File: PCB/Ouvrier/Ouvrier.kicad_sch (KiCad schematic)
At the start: 13 parts, among them J1 Batterie, J2 VBAT Xiao, J3 DC 5V input, Q1 2N2222B, U1 XIAO-ESP32-S3-Plus-DIP, U2 BMP581, U3 UWB

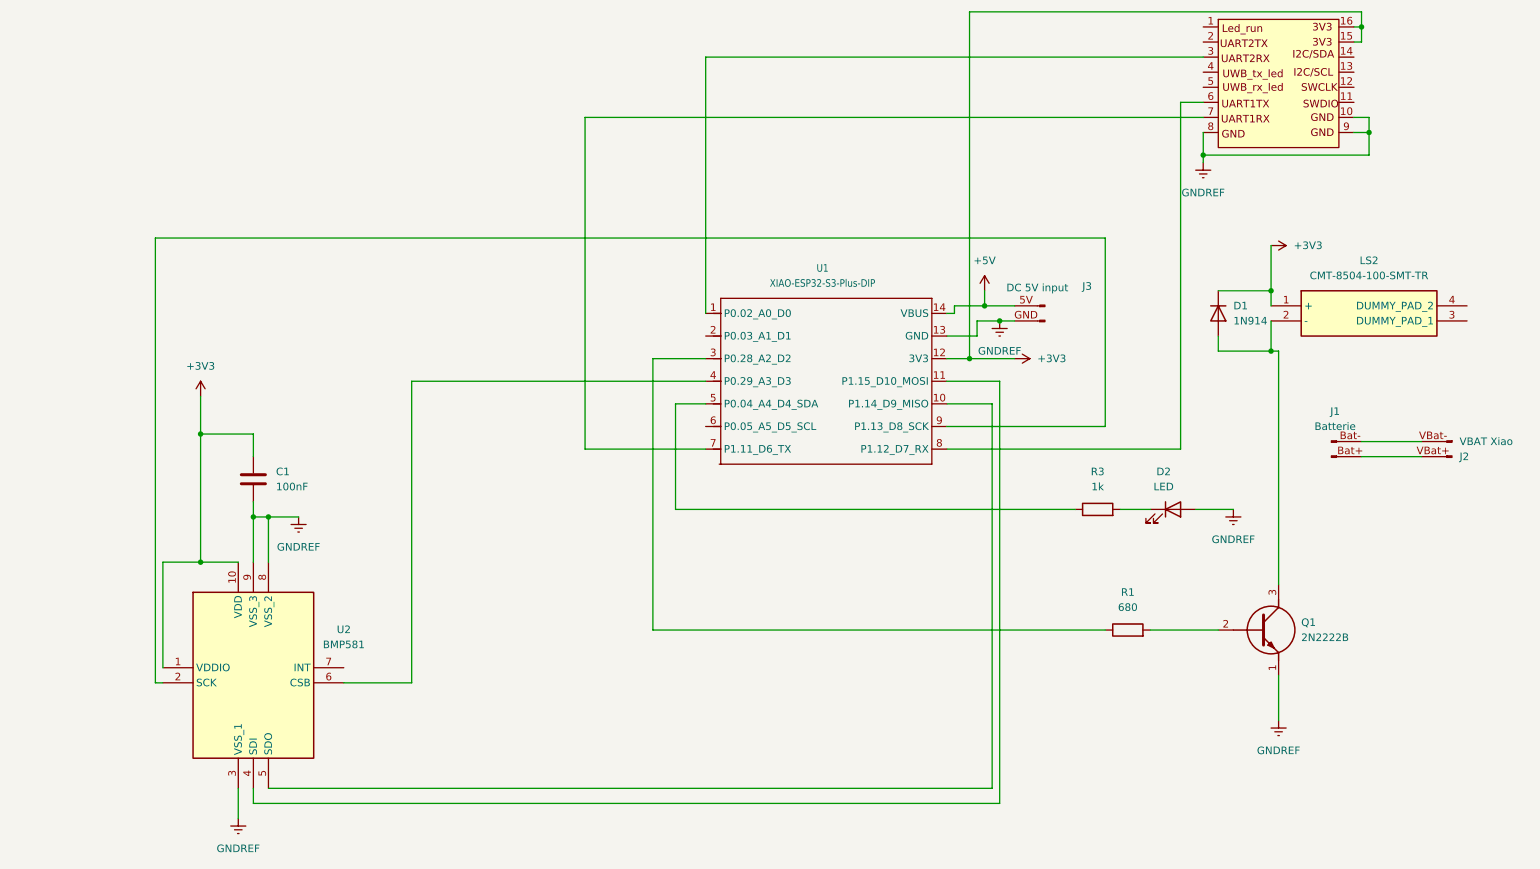
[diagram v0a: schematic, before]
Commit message: Ouvrier_v9_changement_bmp
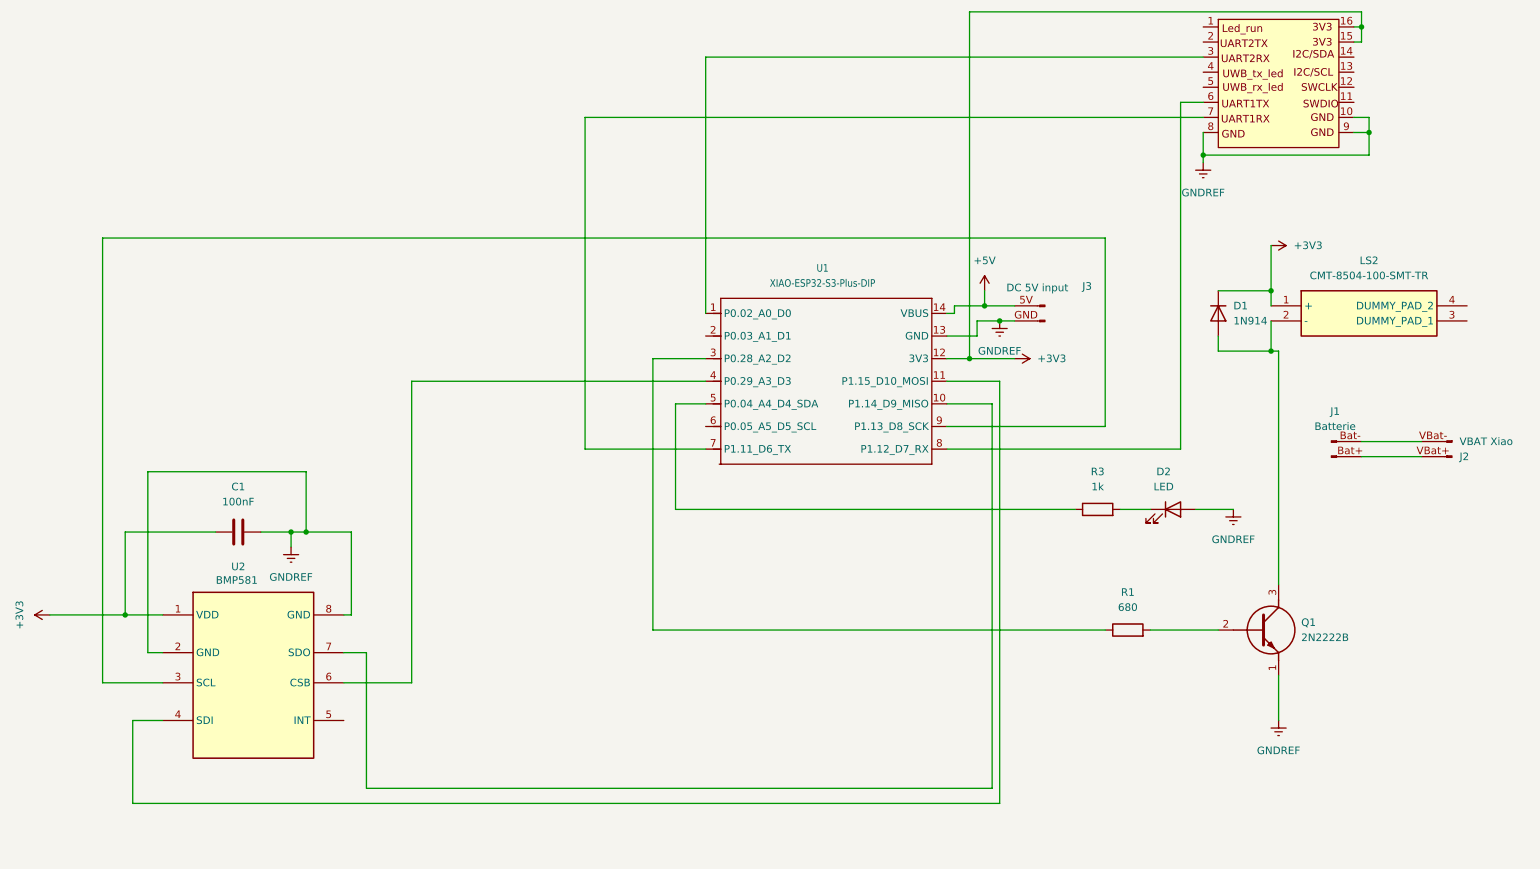
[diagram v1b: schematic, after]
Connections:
- net +3V3: no longer U2.10 (VDD)
- net GNDREF: now also U2.2 (GND); no longer U2.3 (VSS_1), U2.9 (VSS_3)
- net at U1.9 (P1.13_D8_SCK): now also U2.3 (SCL); no longer U2.2 (SCK)
- net at U2.5 (INT): no longer U1.10 (P1.14_D9_MISO)
- net at U2.7 (SDO): now also U1.10 (P1.14_D9_MISO)
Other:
- moved on the sheet: C1

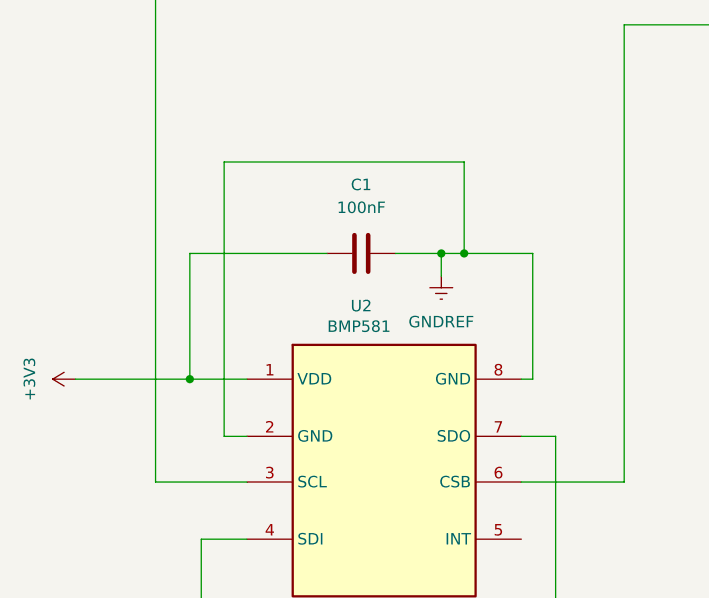
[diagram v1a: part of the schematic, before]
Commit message: Validation sch HUB OUVRIER
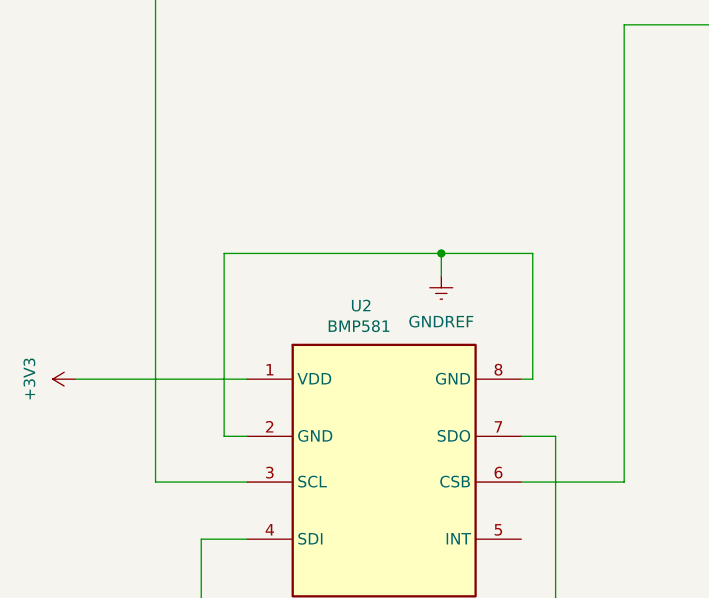
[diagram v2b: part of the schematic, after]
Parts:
- removed C1: 100nF, Capacitor_SMD:C_0402_1005Metric_Pad0.74x0.62mm_HandSolder, symbol Device:C
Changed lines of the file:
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@@
 	)
 	(junction
-		(at 43.18 134.62)
+		(at 251.46 35.56)
 		(diameter 0)
 		(color 0 0 0 0)
@@
 	)
 	(junction
-		(at 251.46 35.56)
-		(diameter 0)
-		(color 0 0 0 0)
-	)
-	(junction
 		(at 236.22 90.17)
 		(diameter 0)
@@
 	)
 	(junction
-		(at 73.66 120.65)
-		(diameter 0)
-		(color 0 0 0 0)
-	)
-	(junction
 		(at 187.96 82.55)
 		(diameter 0)
@@
 	(wire
 		(pts
-			(xy 30.48 134.62) (xy 43.18 134.62)
+			(xy 30.48 134.62) (xy 49.53 134.62)
 		)
 		(stroke
@@
 	(wire
 		(pts
-			(xy 73.66 120.65) (xy 71.12 120.65)
-		)
-		(stroke
-			(width 0)
-			(type default)
-		)
-	)
-	(wire
-		(pts
 			(xy 120.65 106.68) (xy 120.65 50.8)
 		)
@@
 	(wire
 		(pts
-			(xy 58.42 120.65) (xy 43.18 120.65)
-		)
-		(stroke
-			(width 0)
-			(type default)
-		)
-	)
-	(wire
-		(pts
 			(xy 140.97 95.25) (xy 91.44 95.25)
 		)
@@
 	(wire
 		(pts
-			(xy 43.18 134.62) (xy 49.53 134.62)
-		)
-		(stroke
-			(width 0)
-			(type default)
-		)
-	)
-	(wire
-		(pts
-			(xy 66.04 120.65) (xy 71.12 120.65)
-		)
-		(stroke
-			(width 0)
-			(type default)
-		)
-	)
-	(wire
-		(pts
 			(xy 132.08 137.16) (xy 208.28 137.16)
 		)
@@
 	(wire
 		(pts
+			(xy 71.12 120.65) (xy 81.28 120.65)
+		)
+		(stroke
+			(width 0)
+			(type default)
+		)
+	)
+	(wire
+		(pts
 			(xy 250.19 53.34) (xy 252.73 53.34)
 		)
@@
 	(wire
 		(pts
-			(xy 81.28 120.65) (xy 73.66 120.65)
-		)
-		(stroke
-			(width 0)
-			(type default)
-		)
-	)
-	(wire
-		(pts
 			(xy 140.97 40.64) (xy 140.97 83.82)
 		)
@@
 	(wire
 		(pts
-			(xy 46.99 110.49) (xy 73.66 110.49)
+			(xy 46.99 120.65) (xy 71.12 120.65)
 		)
 		(stroke
@@
 	(wire
 		(pts
-			(xy 46.99 140.97) (xy 46.99 110.49)
-		)
-		(stroke
-			(width 0)
-			(type default)
-		)
-	)
-	(wire
-		(pts
-			(xy 43.18 120.65) (xy 43.18 134.62)
+			(xy 46.99 140.97) (xy 46.99 120.65)
 		)
 		(stroke
@@
 		(pts
 			(xy 250.19 35.56) (xy 251.46 35.56)
-		)
-		(stroke
-			(width 0)
-			(type default)
-		)
-	)
-	(wire
-		(pts
-			(xy 73.66 110.49) (xy 73.66 120.65)
 		)
 		(stroke
@@
 					(unit 1)
 				)
-			)
-		)
-	)
-	(symbol
-		(lib_id "Device:C")
-		(at 62.23 120.65 90)
-		(unit 1)
-		(body_style 1)
-		(exclude_from_sim no)
-		(in_bom yes)
-		(on_board yes)
-		(in_pos_files yes)
-		(dnp no)
-		(fields_autoplaced yes)
-		(property "Reference" "C1"
-			(at 62.23 113.03 90)
-			(show_name no)
-			(do_not_autoplace no)
-			(effects
-				(font
-					(size 1.27 1.27)
-				)
-			)
-		)
-		(property "Value" "100nF"
-			(at 62.23 115.57 90)
-			(show_name no)
-			(do_not_autoplace no)
-			(effects
-				(font
-					(size 1.27 1.27)
-				)
-			)
-		)
-		(property "Footprint" "Capacitor_SMD:C_0402_1005Metric_Pad0.74x0.62mm_HandSolder"
-			(at 66.04 119.6848 0)
-			(hide yes)
-			(show_name no)
-			(do_not_autoplace no)
-			(effects
-				(font
-					(size 1.27 1.27)
-				)
-			)
-		)
-		(property "Datasheet" ""
-			(at 62.23 120.65 0)
-			(hide yes)
-			(show_name no)
-			(do_not_autoplace no)
-			(effects
-				(font
-					(size 1.27 1.27)
-				)
-			)
-		)
-		(property "Description" "Unpolarized capacitor"
-			(at 62.23 120.65 0)
-			(hide yes)
-			(show_name no)
-			(do_not_autoplace no)
-			(effects
-				(font
-					(size 1.27 1.27)
-				)
-			)
-		)
-		(pin "1"
-		)
-		(pin "2"
-		)
-		(instances
-			(project "Ouvrier"
-				(path "/84605c1a-5009-408b-9a0f-13132cab7487"
-					(reference "C1")
-					(unit 1)
-				)
